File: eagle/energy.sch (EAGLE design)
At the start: 19 parts, among them J1 S0, J2 NPN, T1 BC547, X1 P1

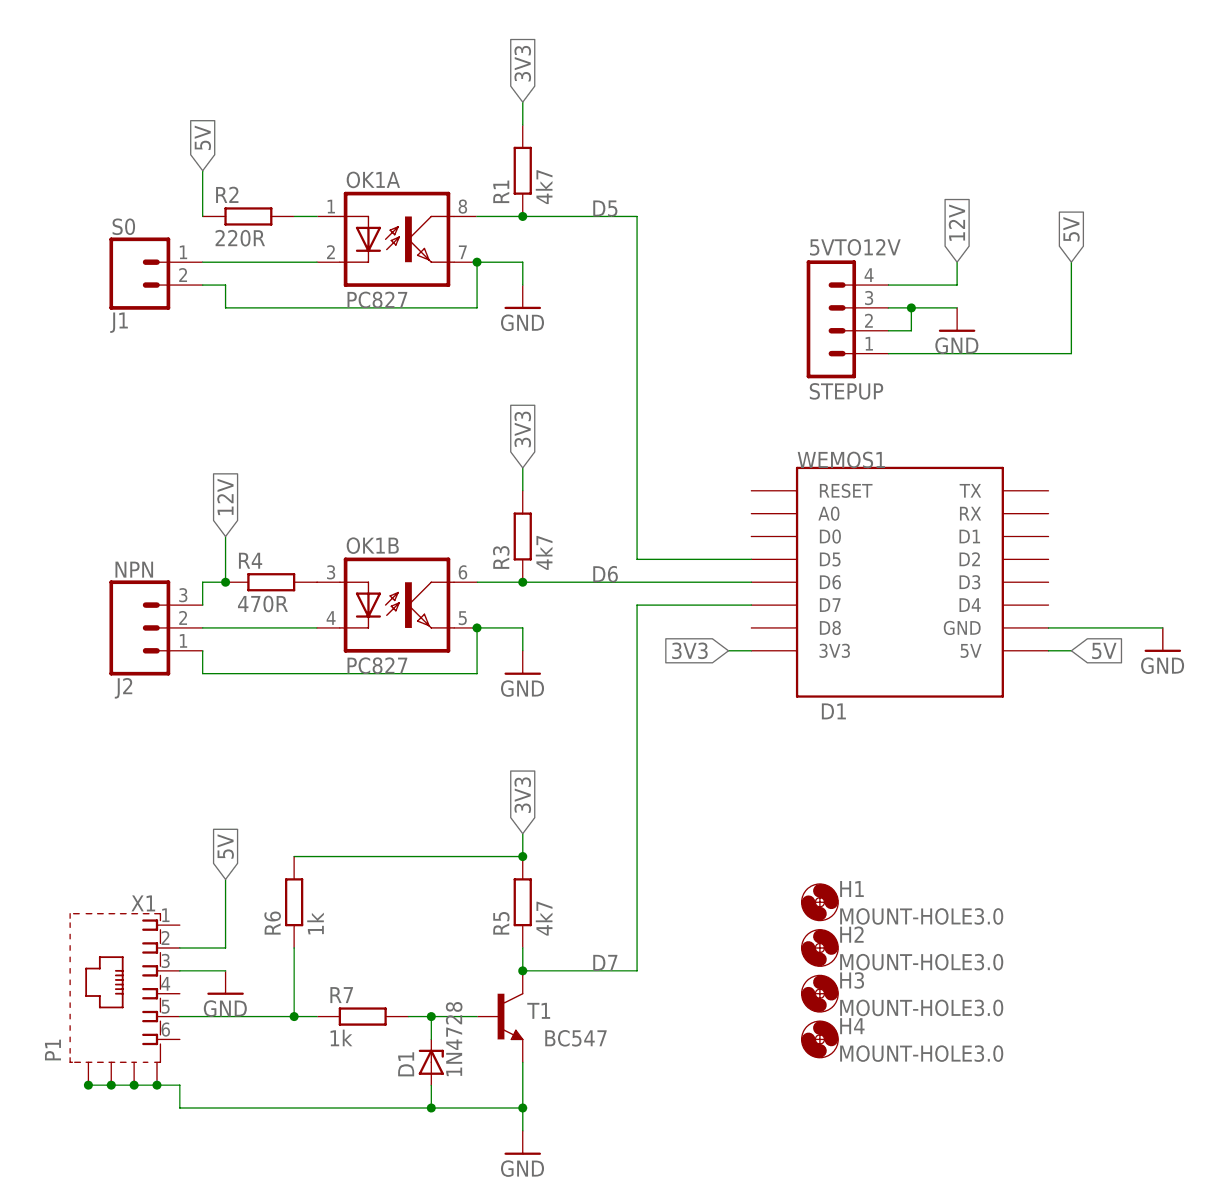
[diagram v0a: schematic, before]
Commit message: Cleaning up
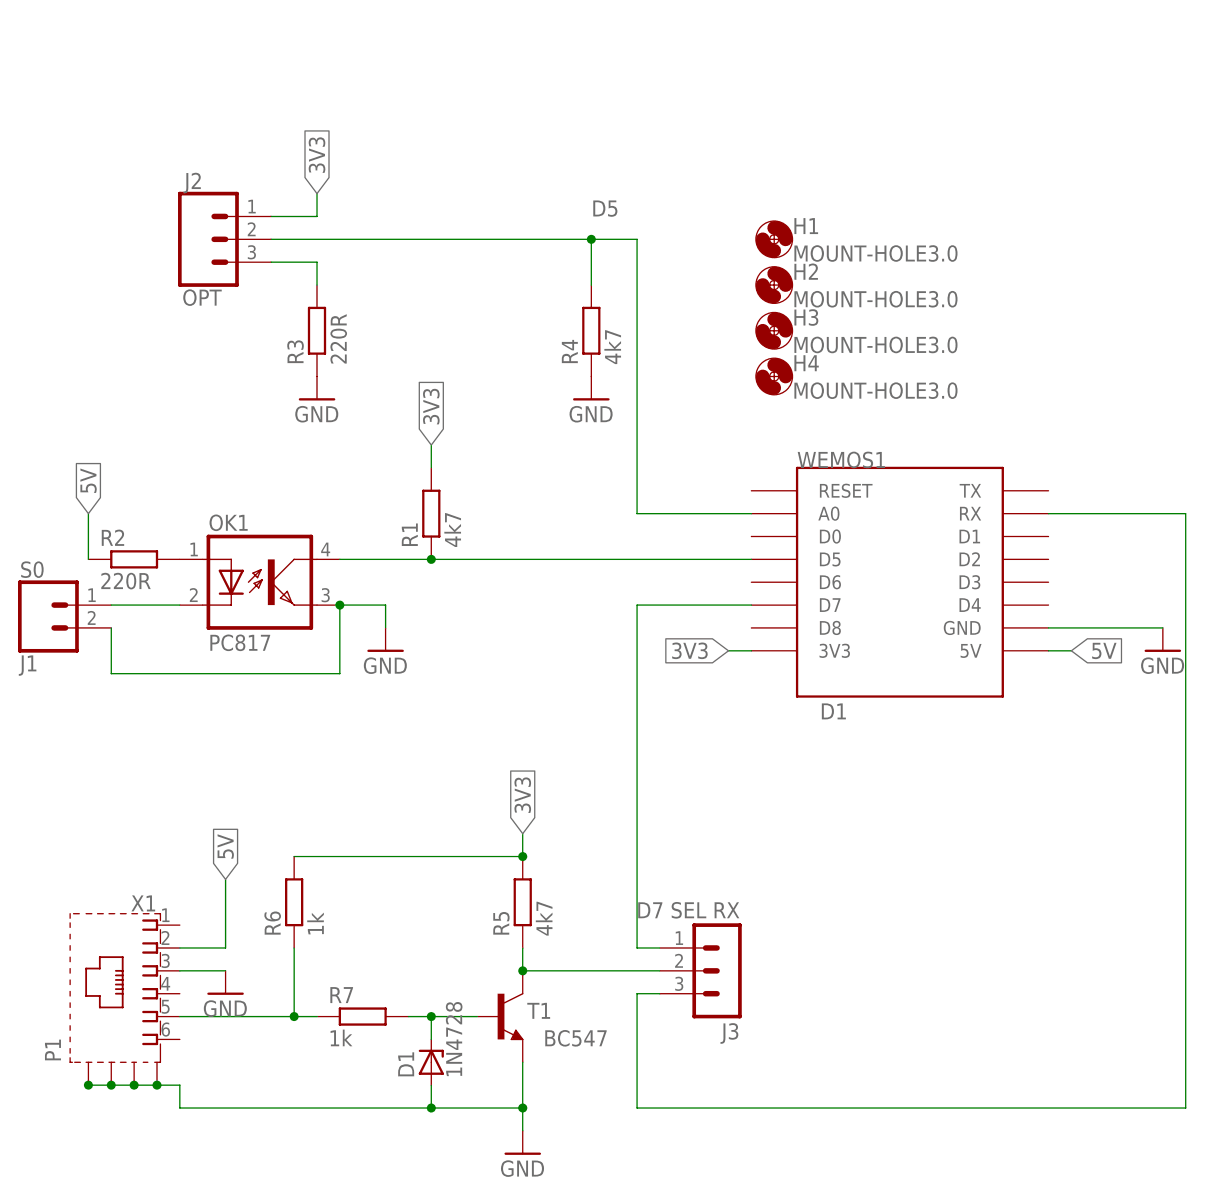
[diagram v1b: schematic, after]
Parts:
- removed 5VTO12V: STEPUP, con-lstb:MA04-1
- added J3: D7 SEL RX, con-lstb:MA03-1
- J2: value NPN -> OPT
- OK1: value PC827 -> PC817; device optocoupler:PC827 -> optocoupler:PC817
- R3: value 4k7 -> 220R
- R4: value 470R -> 4k7
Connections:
- removed net 12V: 5VTO12V.4, J2.3, R4.1
- removed net D6: OK1B.COL, R3.1, WEMOS1.D6
- new net N$5: J3.1, WEMOS1.D7
- new net N$6: J3.3, WEMOS1.RX
- net 3V3: now also J2.1; no longer R3.2
- net 5V: no longer 5VTO12V.1
- net D5: now also OK1.COL; no longer OK1A.COL
- net D7: now also J3.2; no longer WEMOS1.D7
- net GND: now also OK1.EMIT, R3.1, R4.1; no longer 5VTO12V.2, 5VTO12V.3, J2.1, OK1A.EMIT, OK1B.EMIT
- net N$2: now also OK1.C; no longer OK1A.C
- net N$3: now also J2.3, R3.2; no longer OK1B.A, R4.2
- net N$8: now also OK1.A; no longer OK1A.A
- net NPNOUT: now also R4.2, WEMOS1.A0; no longer OK1B.C
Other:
- moved on the sheet: H1, H2, H3, H4, J1, J2, OK1, R1, R2, R3, R4
